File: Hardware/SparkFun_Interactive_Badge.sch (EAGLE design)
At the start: 34 parts, among them Q1 DMG2307L, U1 MIC5205-3.3V, U2 ATMEGA328P, U3 CY7C65213

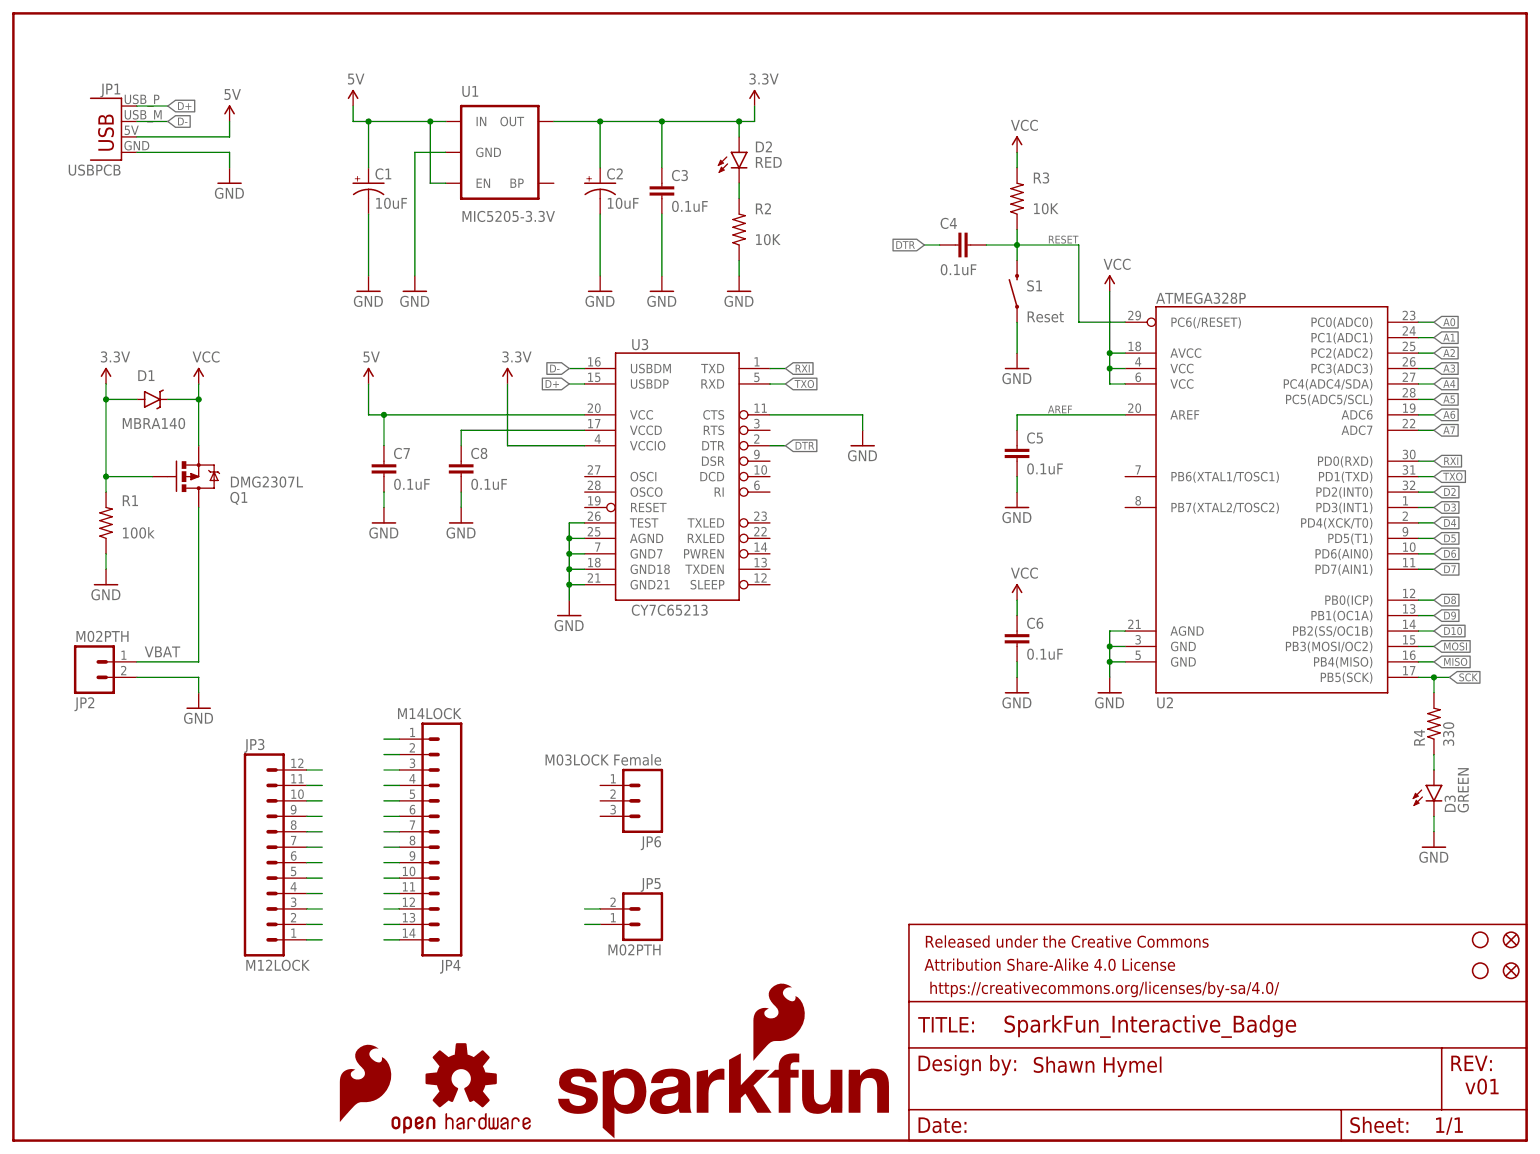
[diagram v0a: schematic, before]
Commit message: Initial layout complete
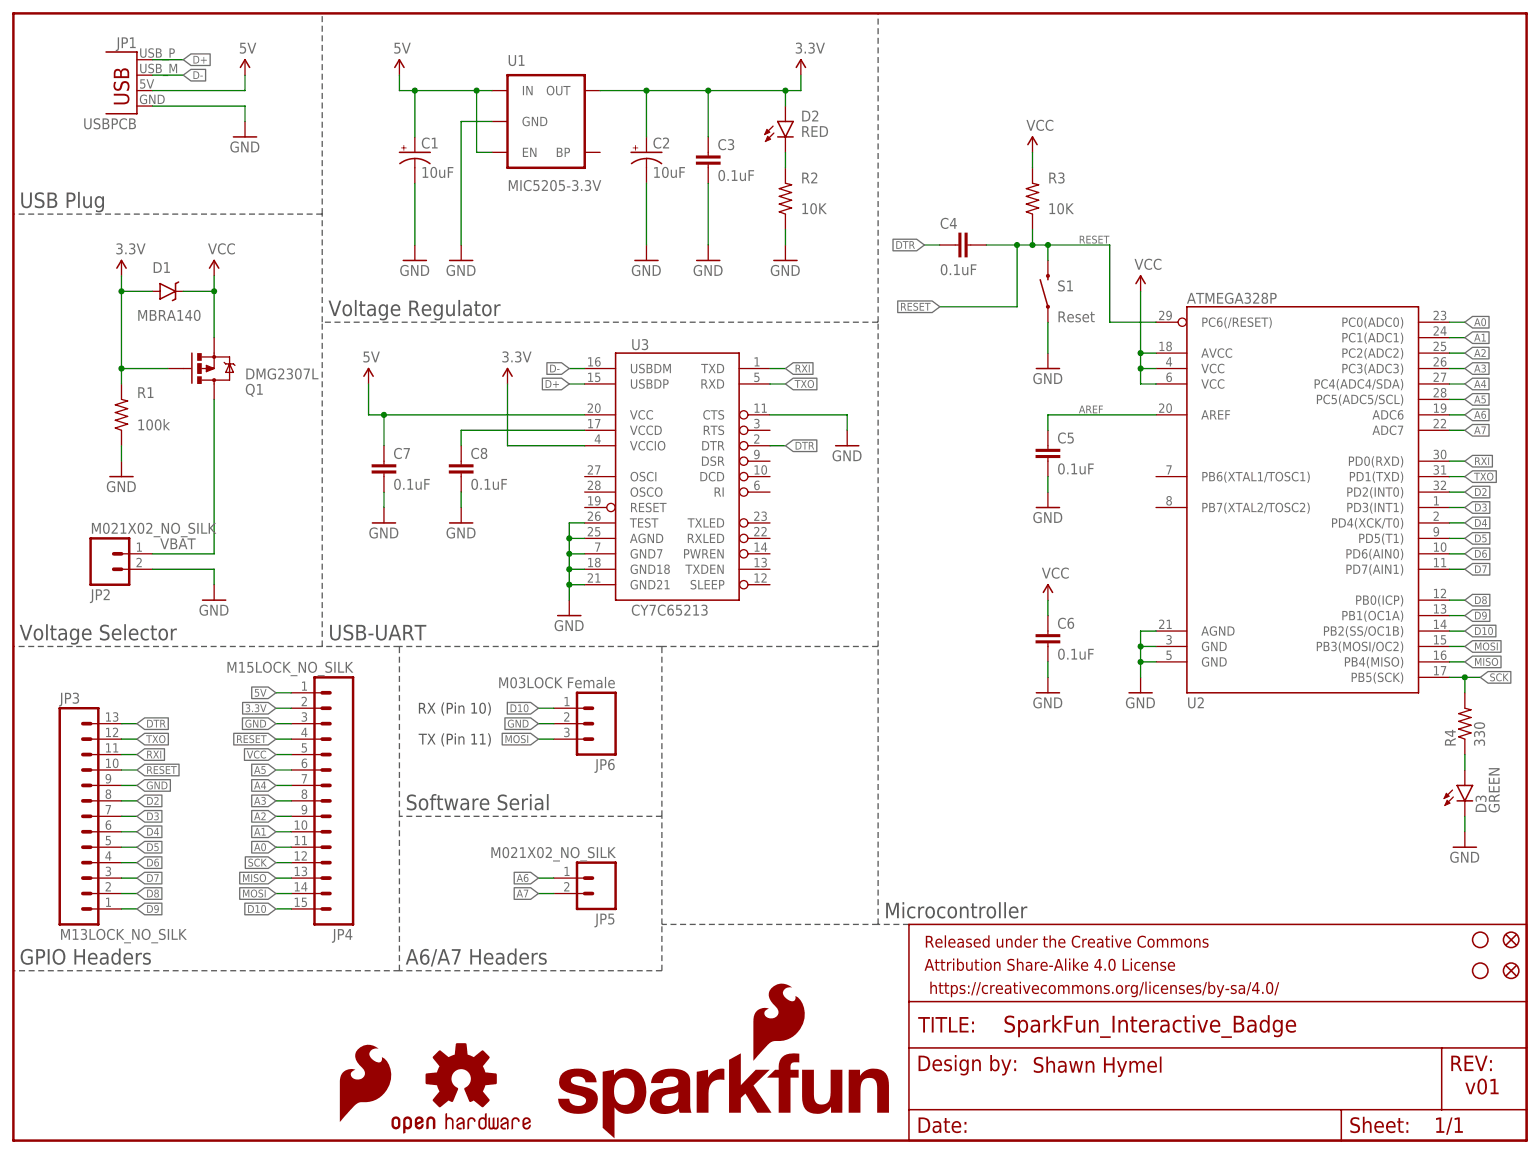
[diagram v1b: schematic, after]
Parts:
- JP2, JP5: value M02PTH -> M021X02_NO_SILK; device SparkFun-Connectors:M02PTH -> SparkFun-Connectors:M021X02_NO_SILK
- JP3: value M12LOCK -> M13LOCK_NO_SILK; device SparkFun-Connectors:M12LOCK -> SparkFun-Connectors:M13LOCK_NO_SILK
- JP4: value M14LOCK -> M15LOCK_NO_SILK; device SparkFun-Connectors:M14LOCK -> SparkFun-Connectors:M15LOCK_NO_SILK
- JP6: device SparkFun-Connectors:M03LOCK -> SparkFun-Connectors:M03LOCK_NO_SILK
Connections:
- removed net N$10: JP3.6
- removed net N$11: JP3.5
- removed net N$12: JP3.4
- removed net N$13: JP3.3
- removed net N$14: JP3.2
- removed net N$15: JP3.1
- removed net N$16: JP4.1
- removed net N$17: JP4.2
- removed net N$18: JP4.3
- removed net N$19: JP4.4
- removed net N$20: JP4.5
- removed net N$21: JP4.6
- removed net N$22: JP4.7
- removed net N$23: JP4.8
- removed net N$24: JP4.9
- removed net N$25: JP4.10
- removed net N$26: JP4.11
- removed net N$27: JP4.12
- removed net N$28: JP4.13
- removed net N$29: JP4.14
- removed net N$3: JP3.12
- removed net N$30: JP5.2
- removed net N$31: JP5.1
- removed net N$5: JP3.11
- removed net N$6: JP3.10
- removed net N$7: JP3.9
- removed net N$8: JP3.8
- removed net N$9: JP3.7
- net 3.3V: now also JP4.2
- net 5V: now also JP4.1
- net A0: now also JP4.11
- net A1: now also JP4.10
- net A2: now also JP4.9
- net A3: now also JP4.8
- net A4: now also JP4.7
- net A5: now also JP4.6
- net A6: now also JP5.1
- net A7: now also JP5.2
- net D10: now also JP4.15, JP6.1
- net D2: now also JP3.8
- net D3: now also JP3.7
- net D4: now also JP3.6
- net D5: now also JP3.5
- net D6: now also JP3.4
- net D7: now also JP3.3
- net D8: now also JP3.2
- net D9: now also JP3.1
- net DTR: now also JP3.13
- net GND: now also JP3.9, JP4.3, JP6.2
- net MISO: now also JP4.13
- net MOSI: now also JP4.14, JP6.3
- net RESET: now also JP3.10, JP4.4
- net RXI: now also JP3.11
- net SCK: now also JP4.12
- net TXO: now also JP3.12
- net VCC: now also JP4.5
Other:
- note added: "A6/A7 Headers"
- note added: "GPIO Headers"
- note added: "Microcontroller"
- note added: "RX (Pin 10)"
- note added: "Software Serial"
- note added: "TX (Pin 11)"
- note added: "USB Plug"
- note added: "USB-UART"
- note added: "Voltage Regulator"
- note added: "Voltage Selector"
- moved on the sheet: C1, C2, C3, C5, C6, D1, D2, D3, JP1, JP2, JP5, JP6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
